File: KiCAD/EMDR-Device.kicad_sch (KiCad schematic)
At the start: 10 parts, among them J1 USB_C_Receptacle_USB2.0_14P, SW1 Switch, U2 ESP32-C6-MINI-1, U6 XC6206PxxxMR

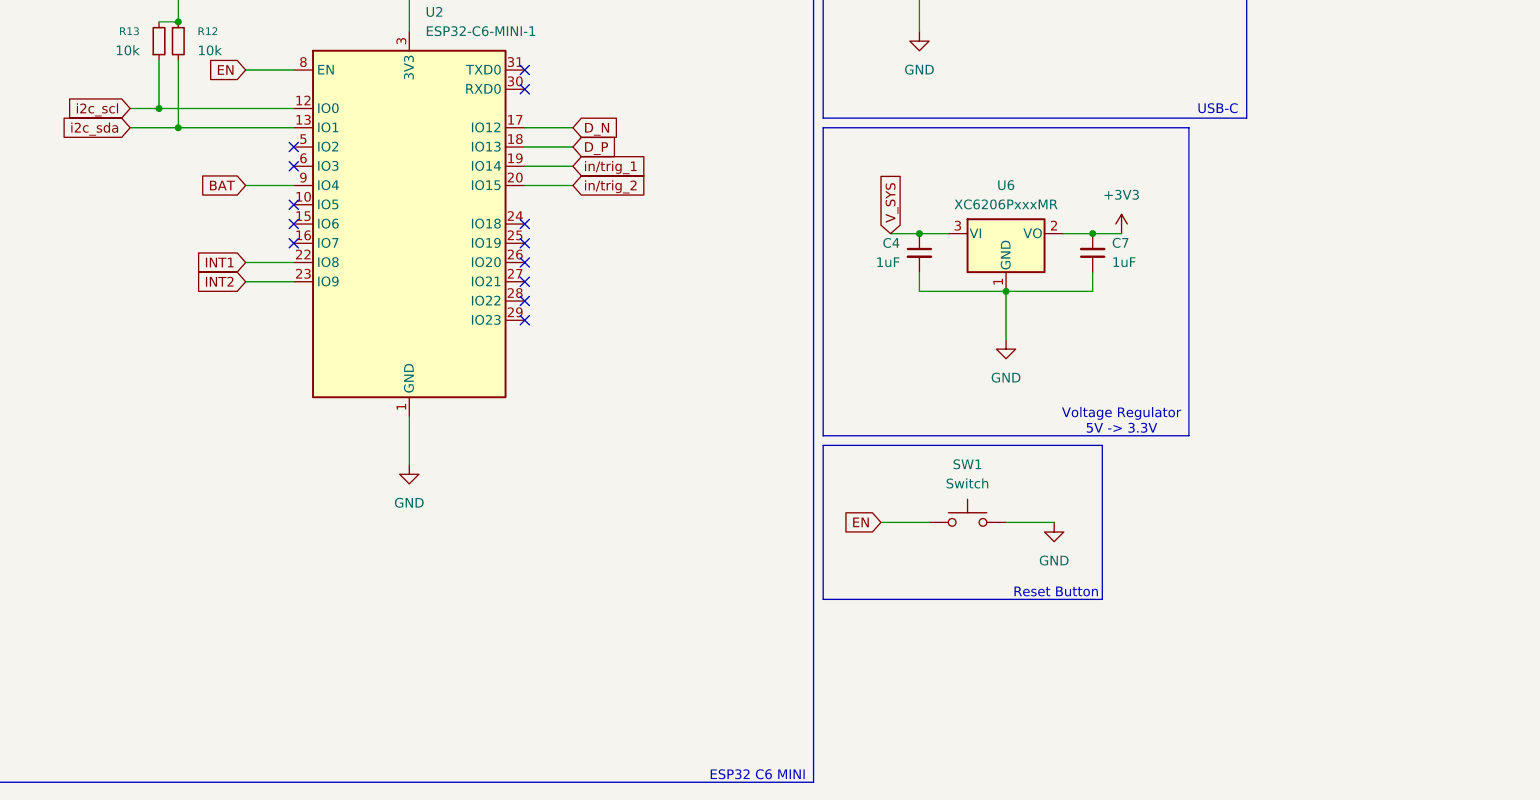
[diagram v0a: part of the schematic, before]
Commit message: preliminary pcb
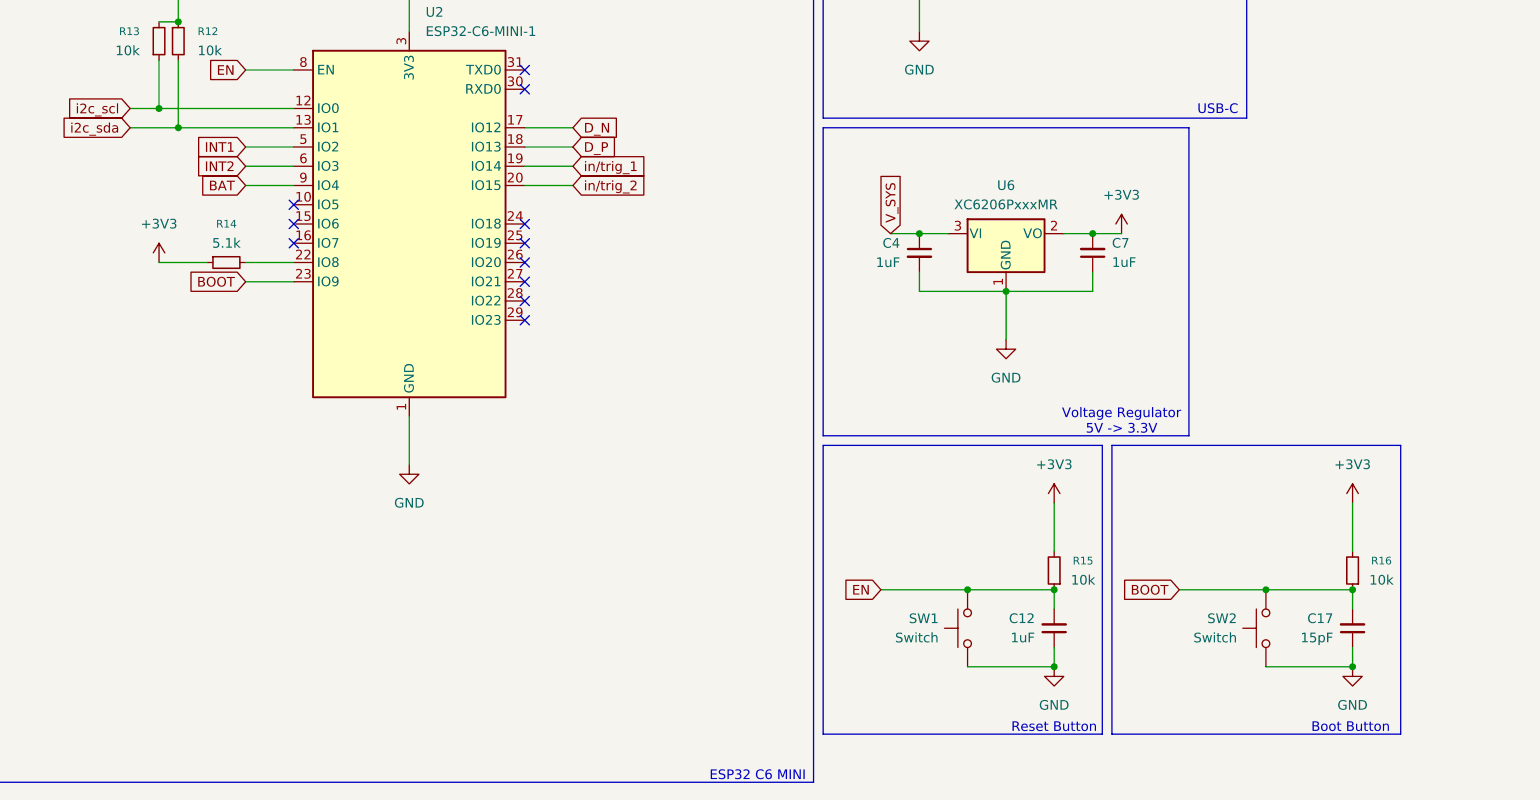
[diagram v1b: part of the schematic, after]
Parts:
- added C12: 1uF, Capacitor_SMD:C_0603_1608Metric, symbol Device:C_Small
- added C17: 15pF, Capacitor_SMD:C_0603_1608Metric, symbol Device:C_Small
- added R14: 5.1k, Resistor_SMD:R_0603_1608Metric, symbol Device:R_Small
- added R15, R16: 10k, Resistor_SMD:R_0603_1608Metric, symbol Device:R_Small
- added SW2: Switch, Button_Switch_SMD:Panasonic_EVQPUJ_EVQPUA, symbol ScottoKeebs:Placeholder_Switch
- SW1: footprint chinh4thepro:reset_switch_smd_side -> Button_Switch_SMD:Panasonic_EVQPUJ_EVQPUA
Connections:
- net +3V3: now also R14.1, R15.2, R16.2
- net EN: now also C12.2, R15.1
- net GND: now also C12.1, C17.1, SW2.2
- net INT1: now also U2.5 (IO2); no longer U2.22 (IO8)
- net INT2: now also U2.6 (IO3); no longer U2.23 (IO9)
- new net: R14.2, U2.22 (IO8)
- new net BOOT: C17.2, R16.1, SW2.1, U2.23 (IO9)
- no-connect marks 13 -> 11
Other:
- note added: "Boot Button"
- moved on the sheet: SW1
